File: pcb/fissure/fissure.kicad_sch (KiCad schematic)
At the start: 27 parts, among them J5 cirque-trackpad, SW3 SW_SPDT, U1 e73-2gm08s1c, U12 e73-2gm08s1c, U4 TLV62568DBV, U5 PMW3610

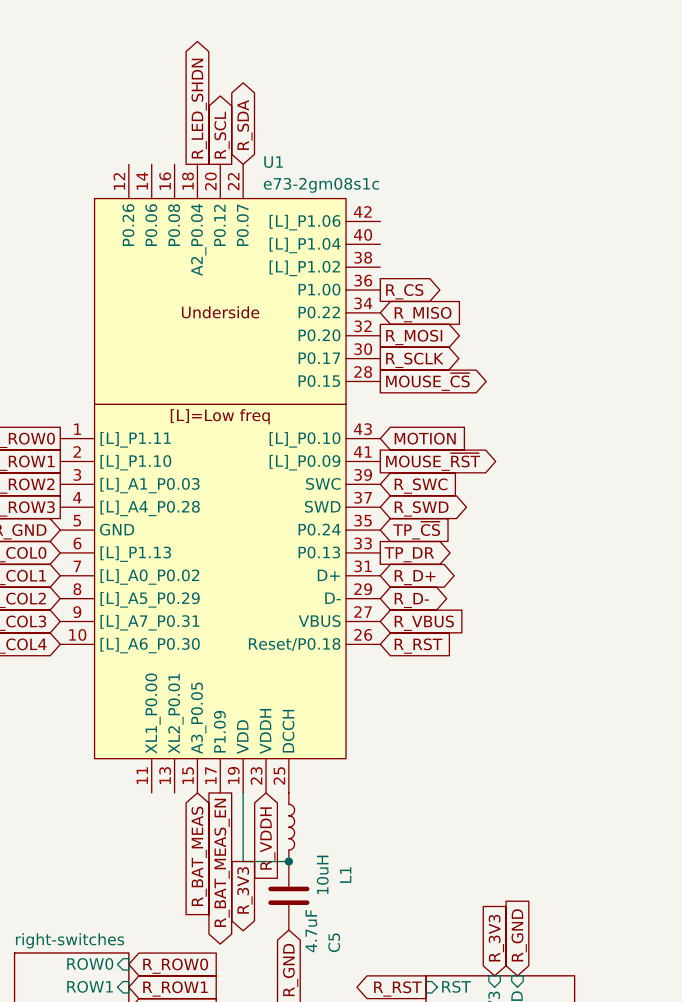
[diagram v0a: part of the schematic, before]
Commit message: break out points
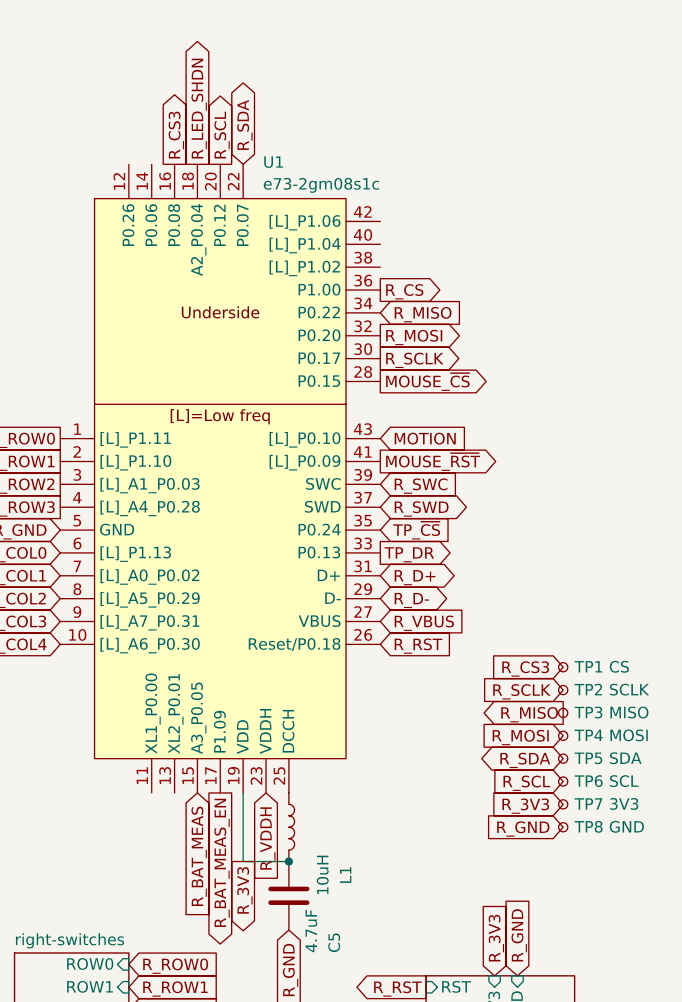
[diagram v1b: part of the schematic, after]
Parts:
- added TP1: CS, TestPoint:TestPoint_THTPad_D1.0mm_Drill0.5mm, symbol Connector:TestPoint_Small
- added TP2: SCLK, TestPoint:TestPoint_THTPad_D1.0mm_Drill0.5mm, symbol Connector:TestPoint_Small
- added TP3: MISO, TestPoint:TestPoint_THTPad_D1.0mm_Drill0.5mm, symbol Connector:TestPoint_Small
- added TP4: MOSI, TestPoint:TestPoint_THTPad_D1.0mm_Drill0.5mm, symbol Connector:TestPoint_Small
- added TP5: SDA, TestPoint:TestPoint_THTPad_D1.0mm_Drill0.5mm, symbol Connector:TestPoint_Small
- added TP6: SCL, TestPoint:TestPoint_THTPad_D1.0mm_Drill0.5mm, symbol Connector:TestPoint_Small
- added TP7: 3V3, TestPoint:TestPoint_THTPad_D1.0mm_Drill0.5mm, symbol Connector:TestPoint_Small
- added TP8: GND, TestPoint:TestPoint_THTPad_D1.0mm_Drill0.5mm, symbol Connector:TestPoint_Small
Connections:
- net GND: now also TP8.1
- net R_3V3: now also TP7.1
- net R_MISO: now also TP3.1
- net R_MOSI: now also TP4.1
- net R_SCL: now also TP6.1
- net R_SCLK: now also TP2.1
- net R_SDA: now also TP5.1
- net R_CS3: now reaches U1.16 (P0.08)
- net R_CS3: now also TP1.1
